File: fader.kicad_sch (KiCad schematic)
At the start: 16 parts, among them J3 QingPu_WQP-PJ366ST, U5 NJM4580

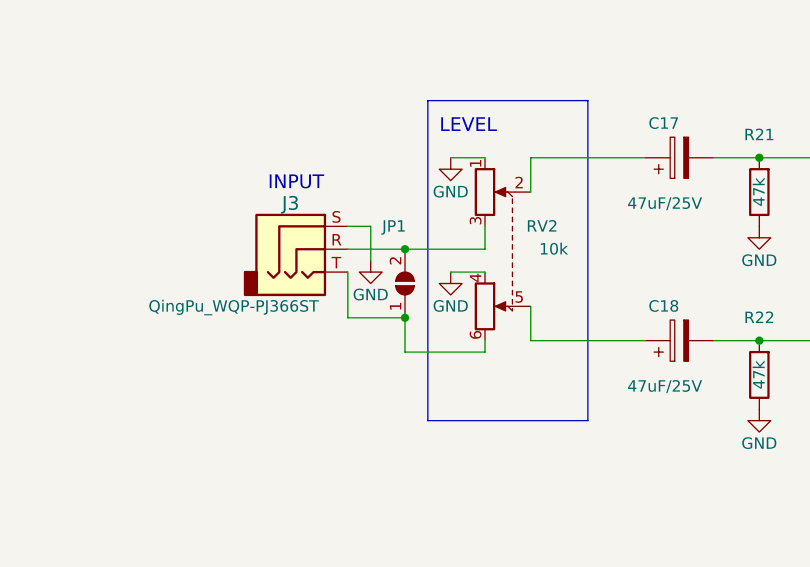
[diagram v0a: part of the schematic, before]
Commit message: update LICENSE
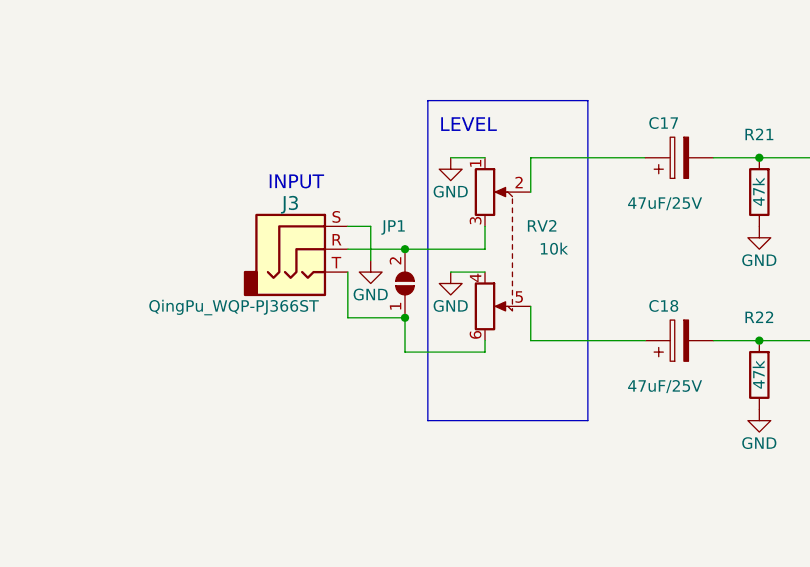
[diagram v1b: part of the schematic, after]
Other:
- company: (none) -> stahllabs
- title: (none) -> mixerli
